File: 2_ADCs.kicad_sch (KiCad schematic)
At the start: 38 parts

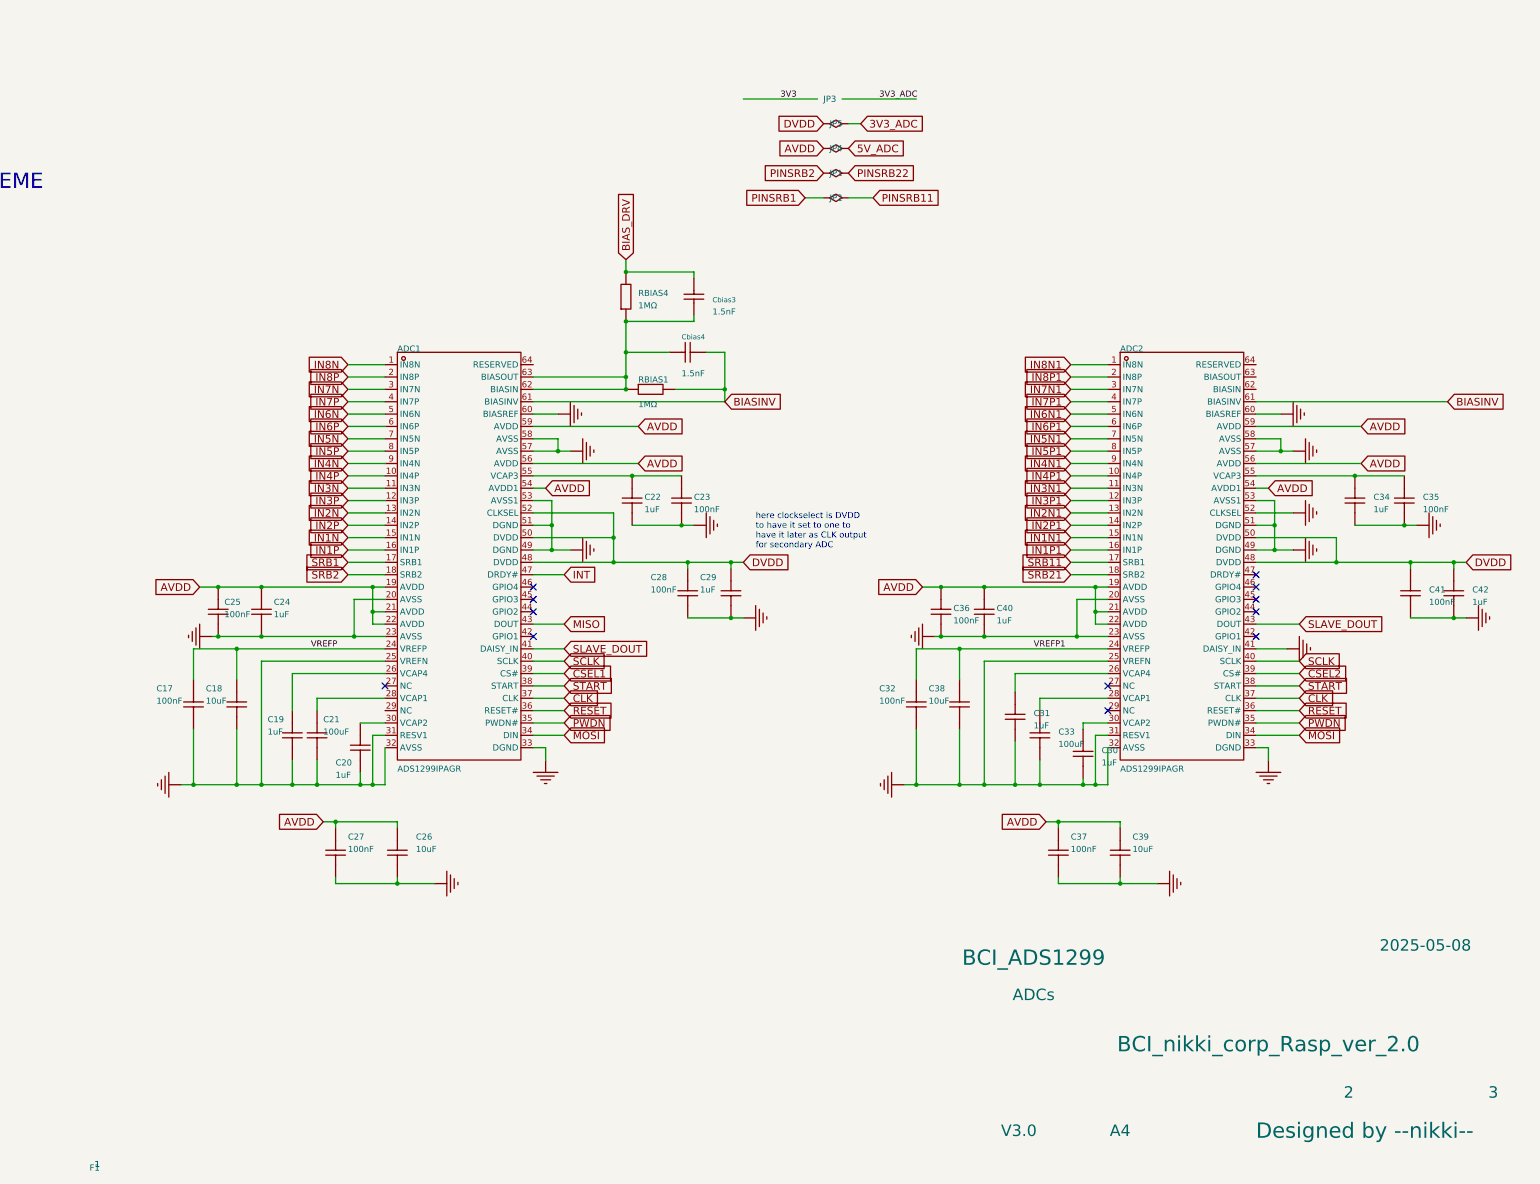
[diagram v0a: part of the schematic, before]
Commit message: Fix ERC
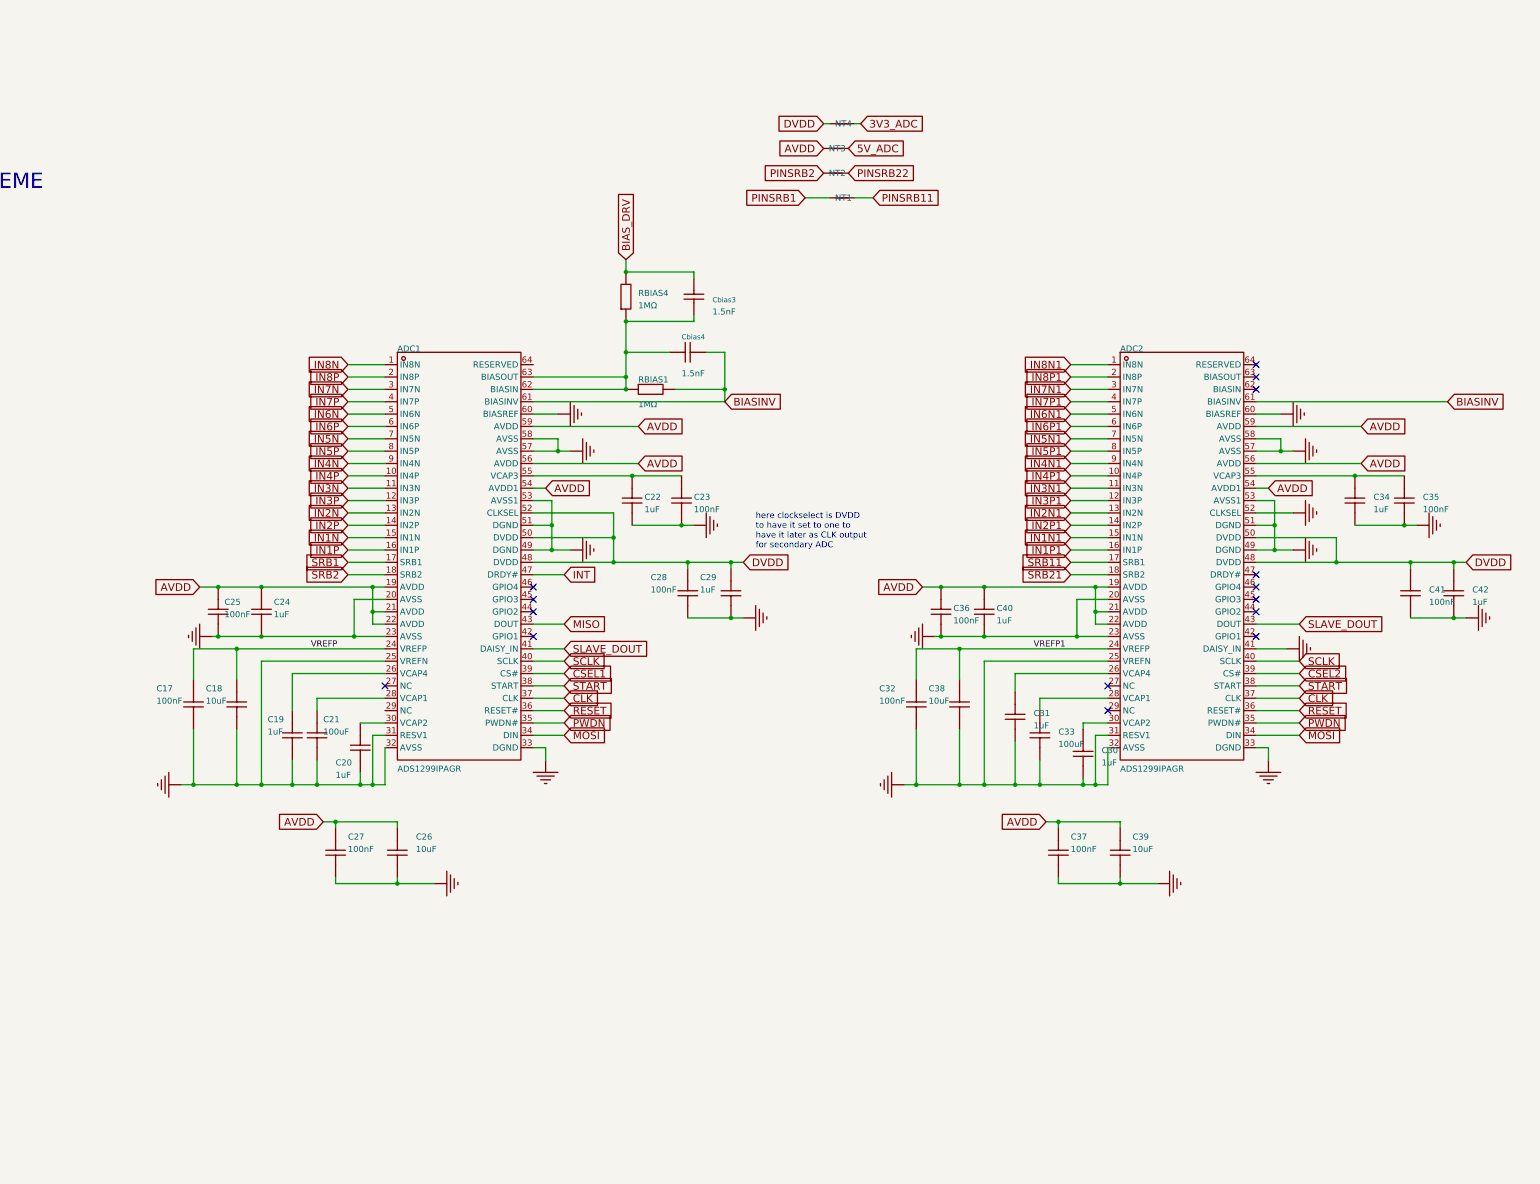
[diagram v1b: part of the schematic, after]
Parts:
- removed F1: (no value), ProPrj_BCI-easyedapro:, symbol ProPrj_BCI-easyedapro:Sheet-Symbol_A4
- removed JP1, JP2, JP4, JP5: (no value), ProPrj_BCI-easyedapro:, symbol ProPrj_BCI-easyedapro:Short-Symbol
- removed JP3: (no value), ProPrj_BCI-easyedapro:, symbol ProPrj_BCI-easyedapro:Short-Symbol-Auto
- added NT1, NT2, NT3, NT4: NetTie_2, symbol Device:NetTie_2
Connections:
- net 3V3_ADC: now also NT4.2
- net 5V_ADC: now also NT3.2
- net AVDD: now also NT3.1
- net DVDD: now also NT4.1
- net PINSRB1: now also NT1.1
- net PINSRB11: now also NT1.2
- net PINSRB2: now also NT2.1
- net PINSRB22: now also NT2.2
- no-connect marks 12 -> 15

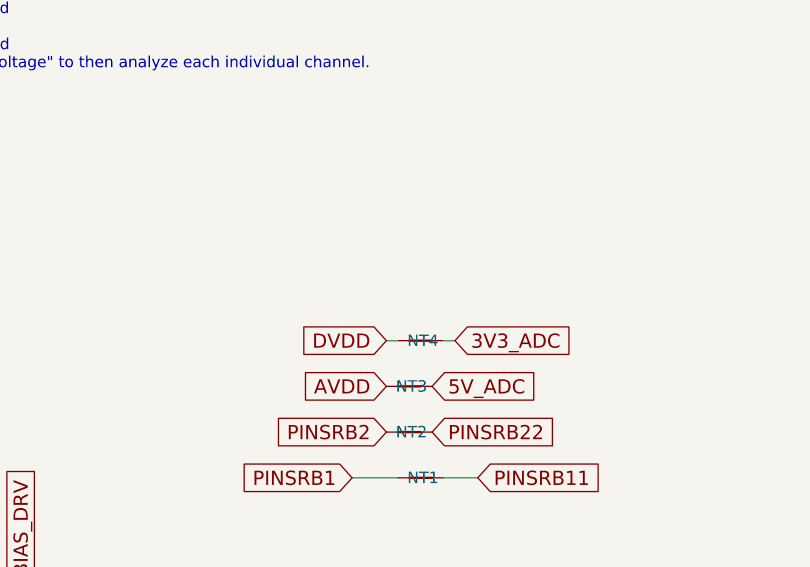
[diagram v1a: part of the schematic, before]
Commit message: PCB update. DRC <300
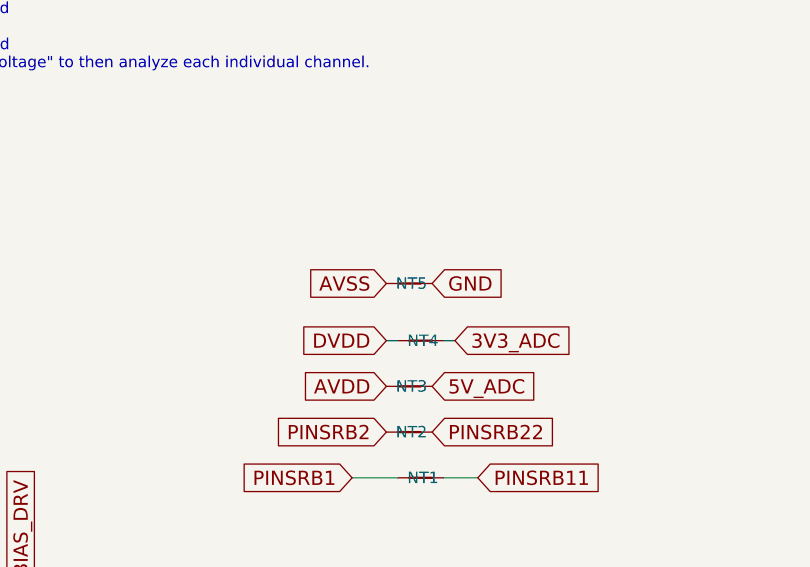
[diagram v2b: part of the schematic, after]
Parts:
- added NT5: NetTie_2, NetTie:NetTie-2_SMD_Pad2.0mm, symbol Device:NetTie_2
- NT1, NT2, NT3, NT4: footprint (none) -> NetTie:NetTie-2_SMD_Pad2.0mm
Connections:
- net GND: now also NT5.2; no longer ADC1.20 (AVSS), ADC1.23 (AVSS), ADC1.25 (VREFN), ADC1.31 (RESV1), ADC1.32 (AVSS), C17.1, C18.1, C19.2, C20.1, C21.2, C24.1, C25.1, C26.1, C27.1
- new net AVSS: ADC1.20 (AVSS), ADC1.23 (AVSS), ADC1.25 (VREFN), ADC1.31 (RESV1), ADC1.32 (AVSS), C17.1, C18.1, C19.2, C20.1, C21.2, C24.1, C25.1, C26.1, C27.1, NT5.1
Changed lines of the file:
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@@
 		)
 	)
+	(global_label "GND"
+		(shape input)
+		(at 242.57 76.2 0)
+		(effects
+			(font
+				(size 1.5748 1.5748)
+			)
+			(justify left)
+		)
+		(property "Intersheetrefs" "${INTERSHEET_REFS}"
+			(at 242.57 76.2 0)
+			(hide yes)
+			(show_name no)
+			(do_not_autoplace no)
+			(effects
+				(font
+					(size 1.27 1.27)
+				)
+			)
+		)
+	)
 	(global_label "AVDD"
 		(shape input)
@@
 		)
 	)
+	(global_label "AVSS"
+		(shape input)
+		(at 237.49 76.2 180)
+		(effects
+			(font
+				(size 1.5748 1.5748)
+			)
+			(justify right)
+		)
+		(property "Intersheetrefs" "${INTERSHEET_REFS}"
+			(at 237.49 76.2 0)
+			(hide yes)
+			(show_name no)
+			(do_not_autoplace no)
+			(effects
+				(font
+					(size 1.27 1.27)
+				)
+			)
+		)
+	)
 	(global_label "AVDD"
 		(shape input)
@@
 	)
 	(symbol
+		(lib_id "Device:NetTie_2")
+		(at 240.03 76.2 0)
+		(unit 1)
+		(body_style 1)
+		(exclude_from_sim no)
+		(in_bom no)
+		(on_board yes)
+		(in_pos_files yes)
+		(dnp no)
+		(property "Reference" "NT5"
+			(at 240.284 76.2 0)
+			(show_name no)
+			(do_not_autoplace no)
+			(effects
+				(font
+					(size 1.27 1.27)
+				)
+			)
+		)
+		(property "Value" "NetTie_2"
+			(at 240.03 77.724 0)
+			(hide yes)
+			(show_name no)
+			(do_not_autoplace no)
+			(effects
+				(font
+					(size 1.27 1.27)
+				)
+			)
+		)
+		(property "Footprint" "NetTie:NetTie-2_SMD_Pad2.0mm"
+			(at 240.03 76.2 0)
+			(hide yes)
+			(show_name no)
+			(do_not_autoplace no)
+			(effects
+				(font
+					(size 1.27 1.27)
+				)
+			)
+		)
+		(property "Datasheet" ""
+			(at 240.03 76.2 0)
+			(hide yes)
+			(show_name no)
+			(do_not_autoplace no)
+			(effects
+				(font
+					(size 1.27 1.27)
+				)
+			)
+		)
+		(property "Description" "Net tie, 2 pins"
+			(at 240.03 76.2 0)
+			(hide yes)
+			(show_name no)
+			(do_not_autoplace no)
+			(effects
+				(font
+					(size 1.27 1.27)
+				)
+			)
+		)
+		(pin "2"
+		)
+		(pin "1"
+		)
+		(instances
+			(project "import2"
+				(path "/06cae45c-d474-473f-93a9-05a684cc4e1b/1b8a5fce-a845-4467-ac27-03cf9cf28f5f"
+					(reference "NT5")
+					(unit 1)
+				)
+			)
+		)
+	)
+	(symbol
 		(lib_id "ProPrj_BCI-easyedapro:GRM188R71H104KA93D")
 		(at 261.62 182.88 90)
@@
 			)
 		)
-		(property "Value" "GND"
+		(property "Value" "AVSS"
 			(at 111.76 187.96 0)
 			(hide yes)
@@
 			)
 		)
-		(property "Footprint" ""
+		(property "Footprint" "NetTie:NetTie-2_SMD_Pad2.0mm"
 			(at 240.03 87.63 0)
 			(hide yes)
@@
 			)
 		)
-		(property "Footprint" ""
+		(property "Footprint" "NetTie:NetTie-2_SMD_Pad2.0mm"
 			(at 240.03 92.71 0)
 			(hide yes)
@@
 			)
 		)
-		(property "Value" "GND"
+		(property "Value" "AVSS"
 			(at 157.48 238.76 0)
 			(hide yes)
@@
 			)
 		)
-		(property "Footprint" ""
+		(property "Footprint" "NetTie:NetTie-2_SMD_Pad2.0mm"
 			(at 241.3 97.79 0)
 			(hide yes)
@@
 			)
 		)
-		(property "Footprint" ""
+		(property "Footprint" "NetTie:NetTie-2_SMD_Pad2.0mm"
 			(at 241.3 82.55 0)
 			(hide yes)
@@
 			)
 		)
-		(property "Value" "GND"
+		(property "Value" "AVSS"
 			(at 105.41 218.44 0)
 			(hide yes)
